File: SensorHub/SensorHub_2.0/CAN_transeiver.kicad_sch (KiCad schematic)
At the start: 4 parts, among them U9 TCAN334

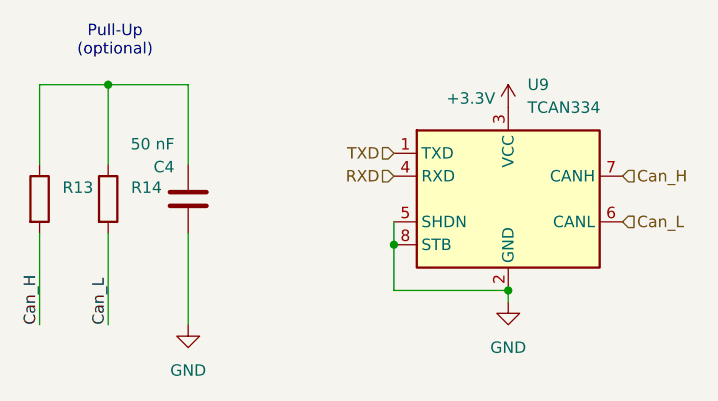
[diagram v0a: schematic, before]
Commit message: TCAN334
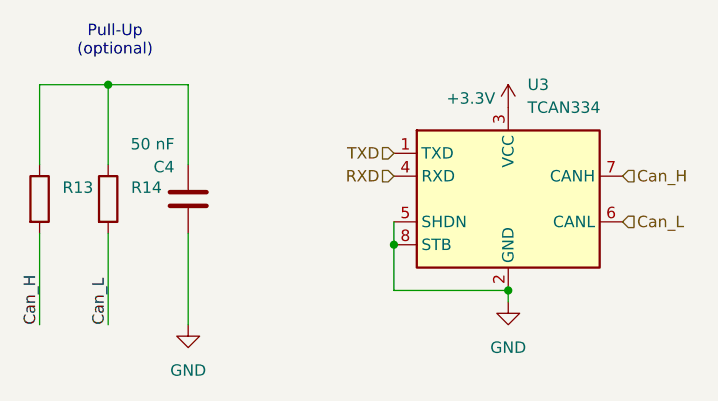
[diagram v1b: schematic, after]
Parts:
- removed U9: TCAN334, Package_TO_SOT_SMD:TSOT-23-8_HandSoldering, symbol Interface_CAN_LIN:TCAN334
- added U3: TCAN334, Package_TO_SOT_SMD:TSOT-23-8, symbol Interface_CAN_LIN:TCAN334
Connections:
- net +3.3V: now also U3.3 (VCC)
- net Can_H: now also U3.7 (CANH)
- net Can_L: now also U3.6 (CANL)
- net GND: now also U3.2 (GND), U3.5 (SHDN), U3.8 (STB)
- net RXD: now also U3.4 (RXD)
- net TXD: now also U3.1 (TXD)
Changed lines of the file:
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@@
+	)
+	(junction
+		(at 118.11 90.17)
+		(diameter 0)
+		(color 0 0 0 0)
+	)
+	(junction
+		(at 149.86 107.95)
+		(diameter 0)
+		(color 0 0 0 0)
 	)
 	(junction
@@
 		(color 0 0 0 0)
 	)
-	(junction
-		(at 149.86 107.95)
-		(diameter 0)
-		(color 0 0 0 0)
-	)
-	(junction
-		(at 118.11 90.17)
-		(diameter 0)
-		(color 0 0 0 0)
-	)
 	(wire
 		(pts
@@
 	(wire
 		(pts
+			(xy 149.86 107.95) (xy 149.86 113.03)
+		)
+		(stroke
+			(width 0)
+			(type default)
+		)
+	)
+	(wire
+		(pts
 			(xy 110.49 90.17) (xy 110.49 99.06)
 		)
@@
 	(wire
 		(pts
+			(xy 127 90.17) (xy 118.11 90.17)
+		)
+		(stroke
+			(width 0)
+			(type default)
+		)
+	)
+	(wire
+		(pts
+			(xy 110.49 116.84) (xy 110.49 106.68)
+		)
+		(stroke
+			(width 0)
+			(type default)
+		)
+	)
+	(wire
+		(pts
+			(xy 162.56 114.3) (xy 162.56 113.03)
+		)
+		(stroke
+			(width 0)
+			(type default)
+		)
+	)
+	(wire
+		(pts
 			(xy 149.86 105.41) (xy 149.86 107.95)
-		)
-		(stroke
-			(width 0)
-			(type default)
-		)
-	)
-	(wire
-		(pts
-			(xy 127 90.17) (xy 118.11 90.17)
-		)
-		(stroke
-			(width 0)
-			(type default)
-		)
-	)
-	(wire
-		(pts
-			(xy 149.86 107.95) (xy 149.86 113.03)
-		)
-		(stroke
-			(width 0)
-			(type default)
-		)
-	)
-	(wire
-		(pts
-			(xy 110.49 116.84) (xy 110.49 106.68)
-		)
-		(stroke
-			(width 0)
-			(type default)
-		)
-	)
-	(wire
-		(pts
-			(xy 162.56 114.3) (xy 162.56 113.03)
 		)
 		(stroke
@@
 	)
 	(symbol
-		(lib_id "Interface_CAN_LIN:TCAN334")
-		(at 162.56 102.87 0)
-		(unit 1)
-		(exclude_from_sim no)
-		(in_bom yes)
-		(on_board yes)
-		(dnp no)
-		(fields_autoplaced yes)
-		(property "Reference" "U9"
-			(at 164.7033 90.17 0)
-			(effects
-				(font
-					(size 1.27 1.27)
-				)
-				(justify left)
-			)
-		)
-		(property "Value" "TCAN334"
-			(at 164.7033 92.71 0)
-			(effects
-				(font
-					(size 1.27 1.27)
-				)
-				(justify left)
-			)
-		)
-		(property "Footprint" "Package_TO_SOT_SMD:TSOT-23-8_HandSoldering"
-			(at 162.56 115.57 0)
-			(effects
-				(font
-					(size 1.27 1.27)
-					(italic yes)
-				)
-				(hide yes)
-			)
-		)
-		(property "Datasheet" "http://www.ti.com/lit/ds/symlink/tcan337.pdf"
-			(at 162.56 102.87 0)
-			(effects
-				(font
-					(size 1.27 1.27)
-				)
-				(hide yes)
-			)
-		)
-		(property "Description" "High-Speed CAN Transceiver, 1Mbps, 3.3V supply, low power standby mode, shutdown mode, SOT-23-8/SOIC-8"
-			(at 162.56 102.87 0)
-			(effects
-				(font
-					(size 1.27 1.27)
-				)
-				(hide yes)
-			)
-		)
-		(pin "4"
-		)
-		(pin "7"
-		)
-		(pin "1"
-		)
-		(pin "5"
-		)
-		(pin "3"
-		)
-		(pin "6"
-		)
-		(pin "8"
-		)
-		(pin "2"
-		)
-		(instances
-			(project "SensorHub_2.0"
-				(path "/9668bc71-8924-498e-982f-628f3083c8b8/aeef27da-d3bb-47bb-8fd5-6871969d5416"
-					(reference "U9")
-					(unit 1)
-				)
-			)
-		)
-	)
-	(symbol
 		(lib_id "Device:R")
 		(at 118.11 102.87 0)
@@
 					(unit 1)
 				)
+			)
+		)
+	)
+	(symbol
+		(lib_id "Interface_CAN_LIN:TCAN334")
+		(at 162.56 102.87 0)
+		(unit 1)
+		(exclude_from_sim no)
+		(in_bom yes)
+		(on_board yes)
+		(dnp no)
+		(fields_autoplaced yes)
+		(property "Reference" "U3"
+			(at 164.7033 90.17 0)
+			(effects
+				(font
+					(size 1.27 1.27)
+				)
+				(justify left)
+			)
+		)
+		(property "Value" "TCAN334"
+			(at 164.7033 92.71 0)
+			(effects
+				(font
+					(size 1.27 1.27)
+				)
+				(justify left)
+			)
+		)
+		(property "Footprint" "Package_TO_SOT_SMD:TSOT-23-8"
+			(at 162.56 115.57 0)
+			(effects
+				(font
+					(size 1.27 1.27)
+					(italic yes)
+				)
+				(hide yes)
+			)
+		)
+		(property "Datasheet" "http://www.ti.com/lit/ds/symlink/tcan337.pdf"
+			(at 162.56 102.87 0)
+			(effects
+				(font
+					(size 1.27 1.27)
+				)
+				(hide yes)
+			)
+		)
+		(property "Description" "High-Speed CAN Transceiver, 1Mbps, 3.3V supply, low power standby mode, shutdown mode, SOT-23-8/SOIC-8"
+			(at 162.56 102.87 0)
+			(effects
+				(font
+					(size 1.27 1.27)
+				)
+				(hide yes)
+			)
+		)
+		(pin "3"
+		)
+		(pin "5"
+		)
+		(pin "1"
+		)
+		(pin "4"
+		)
+		(pin "2"
+		)
+		(pin "8"
+		)
+		(pin "7"
+		)
+		(pin "6"
+		)
+		(instances
+			(project "SensorHub_2.0"
+				(path "/9668bc71-8924-498e-982f-628f3083c8b8/aeef27da-d3bb-47bb-8fd5-6871969d5416"
+					(reference "U3")
+					(unit 1)
+				)
